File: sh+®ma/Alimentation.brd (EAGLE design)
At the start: 171.4 x 101.3 mm, 17 parts, among them X1 87758-4016

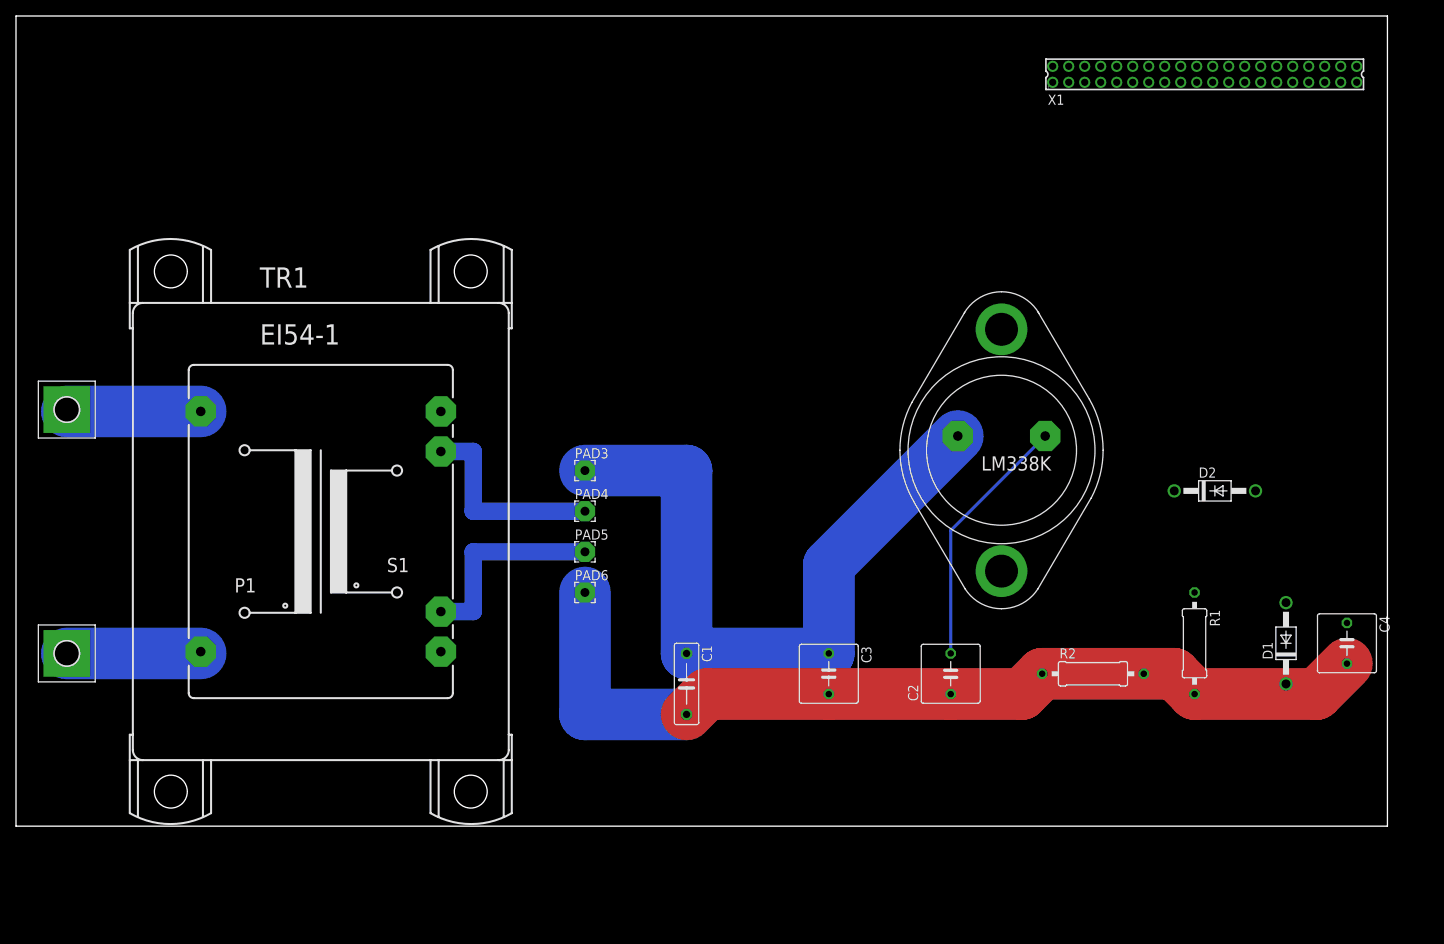
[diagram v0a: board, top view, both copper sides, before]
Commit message: Carte mère (résolution problème transfo)
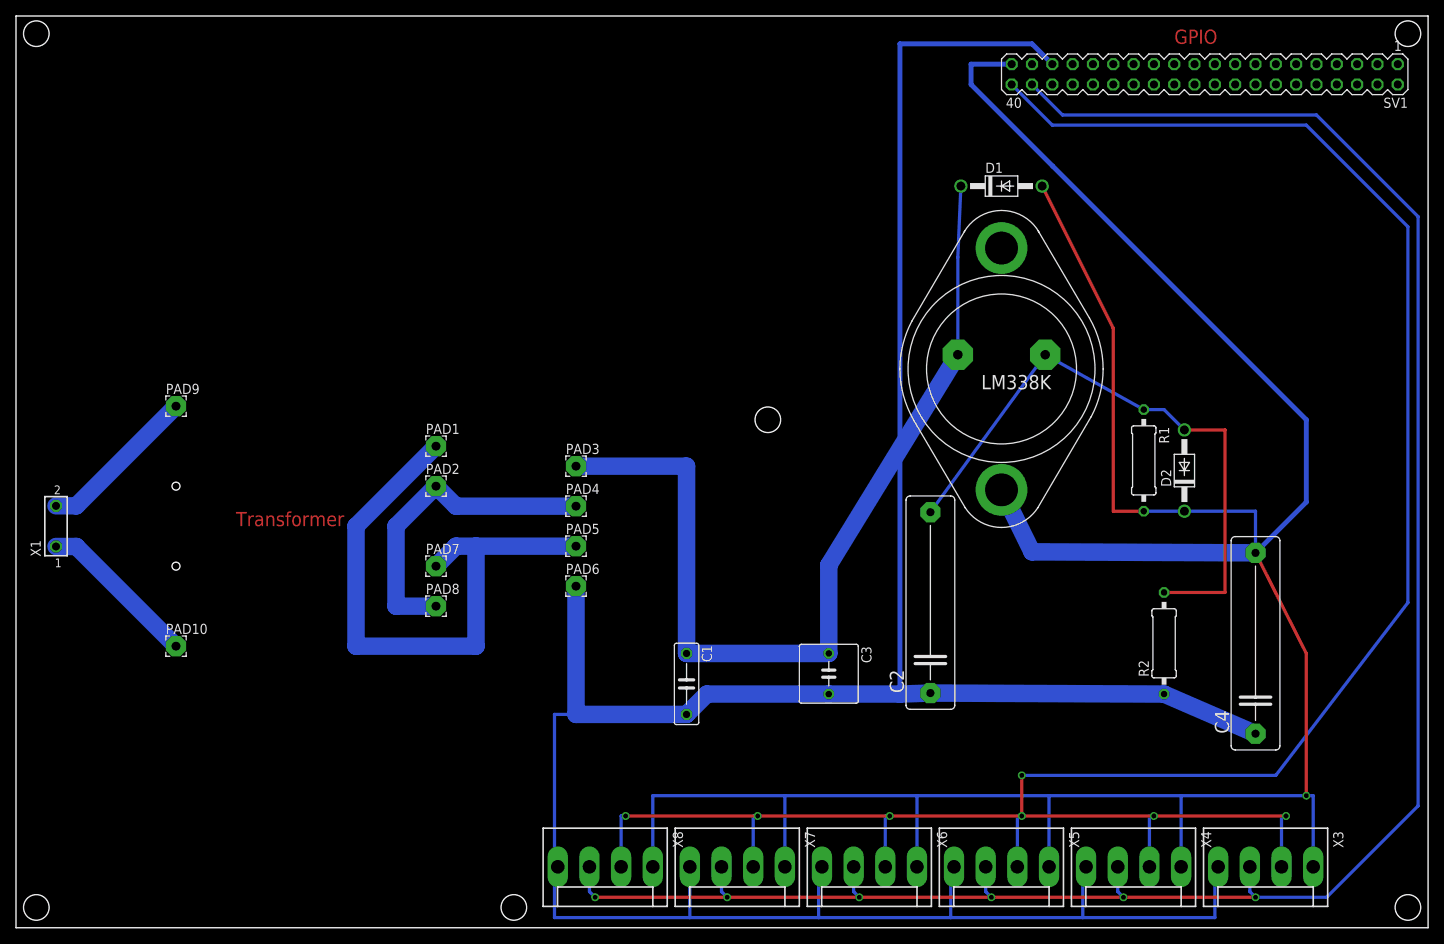
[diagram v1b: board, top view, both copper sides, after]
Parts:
- removed H1, H2: MOUNT-PAD-SQUARE3.0, holes:3,0-PAD-SQUARE
- removed TR1: (no value), trafo:EI54-1B
- added PAD1, PAD10, PAD2, PAD7, PAD8, PAD9: (no value), wirepad:2,54/1,1
- added SV1: (no value), con-lstb:MA20-2
- added X3, X4, X5, X6, X7, X8: (no value), con-molex:KK-156-4
- C2, C4: device rcl:C050-075X075 -> capacitor-wima:C22.5B6
- X1: value 87758-4016 -> TSW-101-02-S-Q; device con-molex:87758-4016 -> con-samtec:TSW-101-02-S-Q
- moved X1 154.3 mm to (5.00, 37.5)
- moved D1 67.3 mm to (123.2, 80.0), turned to 0 degrees
- moved R1 23.7 mm to (141.0, 45.7)
- moved C4 11.4 mm to (154.9, 22.9), turned to 90 degrees
- moved LM338K 10.2 mm to (123.2, 57.1)
- moved R2 9.67 mm to (143.5, 22.9), turned to 90 degrees
- moved C2 9.25 mm to (114.3, 27.9)
- moved D2 4.58 mm to (146.1, 44.5), turned to 90 degrees
- moved PAD6 1.37 mm to (70.0, 30.0)
- moved PAD5 1.33 mm to (70.0, 35.0)
- moved PAD4 1.29 mm to (70.0, 40.0)
- moved PAD3 1.25 mm to (70.0, 45.0)
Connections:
- removed net N$8 (its old number): C4.2, D1.A, D2.C, LM338K.3, R1.2, X1.2
- new net N$10: C4.2, D1.A, D2.C, LM338K.3, R1.2, SV1.39, X3.1, X4.1, X5.1, X6.1, X7.1, X8.1
- new net N$7: SV1.38, X3.3, X4.3, X5.3, X6.3, X7.3, X8.3
- new net N$9: SV1.40, X3.2, X4.2, X5.2, X6.2, X7.2, X8.2
- net N$1: now also PAD9.1, X1.2; no longer PAD4.1, TR1.13
- net N$2: now also PAD10.1, X1.1; no longer PAD5.1, TR1.9
- net N$3: now also SV1.35, X3.4, X4.4, X5.4, X6.4, X7.4, X8.4; no longer X1.6
- net N$5: now also PAD2.1, PAD4.1, PAD8.1; no longer H1.B3,0, TR1.1
- net N$6: now also PAD1.1, PAD5.1, PAD7.1; no longer H2.B3,0, TR1.7
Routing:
- net N$10: track 0.00 -> 356.2 mm, vias 0 -> 1
- net N$9: track 0.00 -> 291.9 mm, vias 0 -> 7
- net N$7: track 0.00 -> 261.0 mm, vias 0 -> 6
- net N$3: track 94.6 -> 350.4 mm
- net N$6: track 17.0 -> 75.2 mm
- net N$8: track 32.1 -> 77.6 mm
- net N$4: track 87.2 -> 118.0 mm
- net N$5: track 17.0 -> 40.6 mm
- net N$8 (its old number): track 20.6 -> 0.00 mm
- net N$1: track 26.7 -> 20.2 mm
- net N$2: track 25.5 -> 20.2 mm
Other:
- board size 171.4 x 101.3 mm -> 176.5 x 114 mm
- board text added: "GPIO"
- board text added: "Transformer"
